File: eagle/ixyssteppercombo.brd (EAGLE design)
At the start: 152.7 x 152.4 mm, 47 parts, among them K1 G5V-2, X4 BU-SMA-V

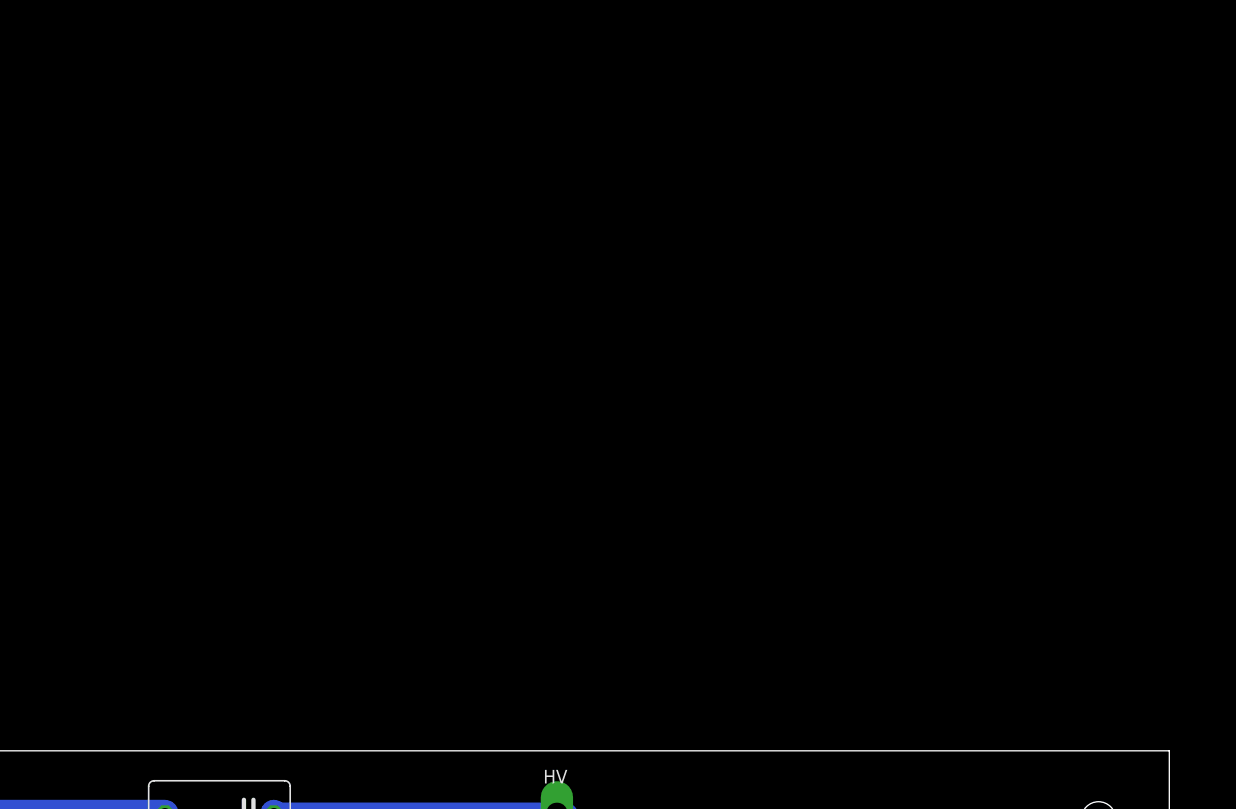
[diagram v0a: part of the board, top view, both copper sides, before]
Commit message: IXYS board solution, gatedriver components
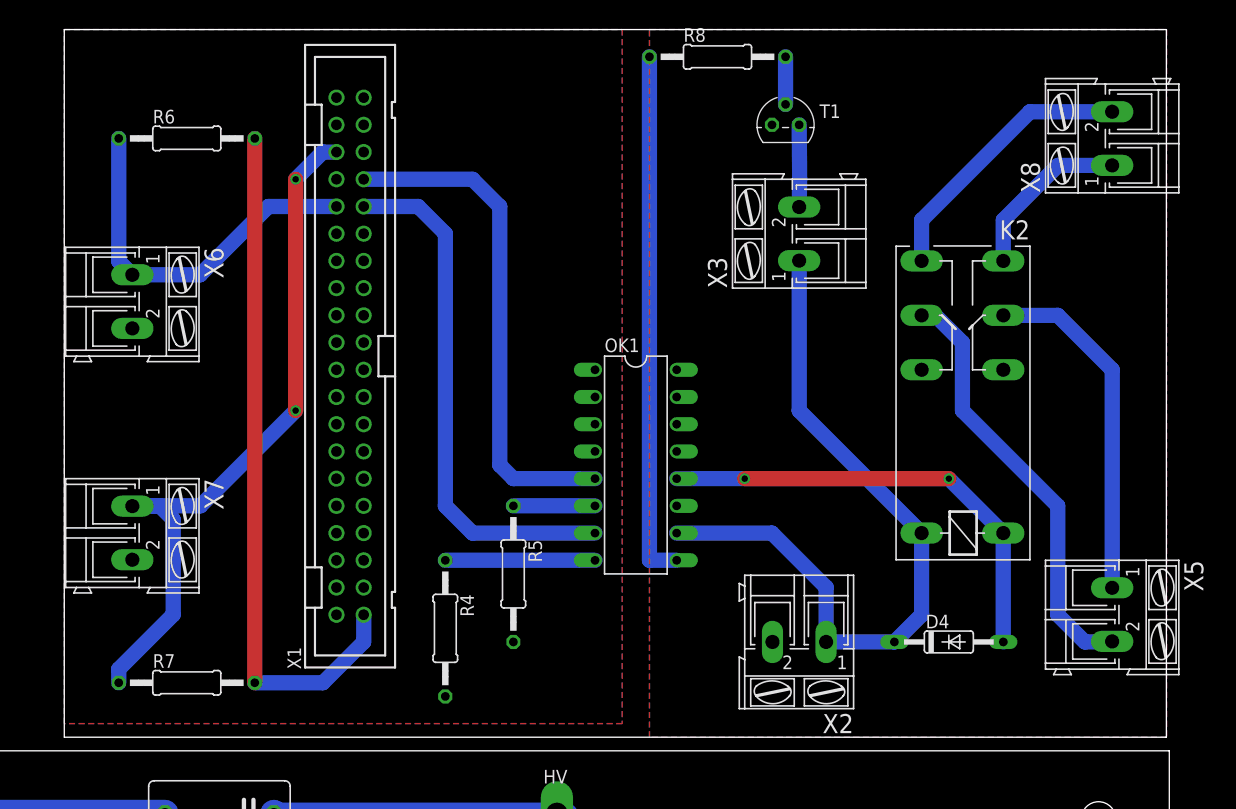
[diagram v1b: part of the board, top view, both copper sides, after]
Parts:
- added D4: 1N4148DO35-10, diode:DO35-10
- added K2: RP420005, relay:RP420
- added OK1: PS2501", optocoupler:DIL16
- added R4, R5: 200, resistor:0207/12
- added R6, R7: 1k, resistor:0207/12
- added R8: (no value), rcl:0207/12
- added T1: 2N3904, transistor:TO92
- added X1: 2540-, con-3m:PAK100/2500-40
- added X2, X3, X5, X6, X7, X8: (no value), con-ptr500:AK300/2
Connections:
- new net +24V: D4.C, K2.A2, OK1.10, X2.1, X3.1
- new net +3V3: R6.2, R7.2, X1.1, X1.17
- new net +5V: X1.2, X1.4
- new net GND1: R4.2, R5.2, X1.14, X1.20, X1.25, X1.30, X1.34, X1.39, X1.6, X1.9, X6.2, X7.2
- new net GND2: OK1.11, T1.3, X2.2
- new net GPIO13: OK1.5, X1.33
- new net GPIO19: X1.35
- new net GPIO20: X1.38
- new net GPIO21: X1.40
- new net GPIO26: X1.37
- new net GPIO5: X1.29
- new net GPIO6: OK1.7, X1.31
- new net N$13: X1.3
- new net N$20: X1.5
- new net N$22: X1.8
- new net N$23: X1.10
- new net N$24: X1.19
- new net N$26: X1.21
- new net N$27: X1.23
- new net N$28: X1.24
- new net N$29: X1.26
- new net N$30: X1.27
- new net N$31: X1.28
- new net N$32: OK1.8, R4.1
- new net N$33: OK1.6, R5.1
- new net N$34: R6.1, X1.32, X6.1
- new net N$35: D4.A, K2.A1, OK1.12
- new net N$36: X1.36, X7.1
- new net N$37: R7.1, X7.1
- new net N$38: OK1.9, R8.1
- new net N$39: T1.1, X3.2
- new net N$40: R8.2, T1.2
- new net N$41: K2.11, X5.1
- new net N$42: K2.14, X8.1
- new net N$43: K2.21, X5.2
- new net N$44: K2.24, X8.2
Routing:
- net +24V: track 0.00 -> 68.9 mm
- net +3V3: track 0.00 -> 65.1 mm
- net N$38: track 0.00 -> 49.5 mm
- net GPIO6: track 0.00 -> 49.1 mm
- net GPIO13: track 0.00 -> 47.3 mm
- net N$36: track 0.00 -> 45.4 mm, vias 0 -> 2
- net N$35: track 0.00 -> 42.7 mm, vias 0 -> 2
- net N$43: track 0.00 -> 40.1 mm
- net N$34: track 0.00 -> 34.9 mm
- net N$41: track 0.00 -> 32.6 mm
- net N$44: track 0.00 -> 25.8 mm
- net N$37: track 0.00 -> 21.7 mm
- net N$42: track 0.00 -> 16.1 mm
- net N$32: track 0.00 -> 14.0 mm
- net N$39: track 0.00 -> 7.67 mm
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- added copper zone on layer 1, net GND1
- added copper zone on layer 16, net GND1
- added copper zone on layer 1, net GND2
- added copper zone on layer 16, net GND2
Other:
- board size 152.7 x 152.4 mm -> 152.7 x 219.7 mm
